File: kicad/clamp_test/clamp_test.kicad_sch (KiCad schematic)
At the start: 26 parts, among them J1 Conn_Coaxial, J2 Conn_Coaxial, J3 Conn_01x03_Pin, J4 Conn_Coaxial, U1 LT1365CS

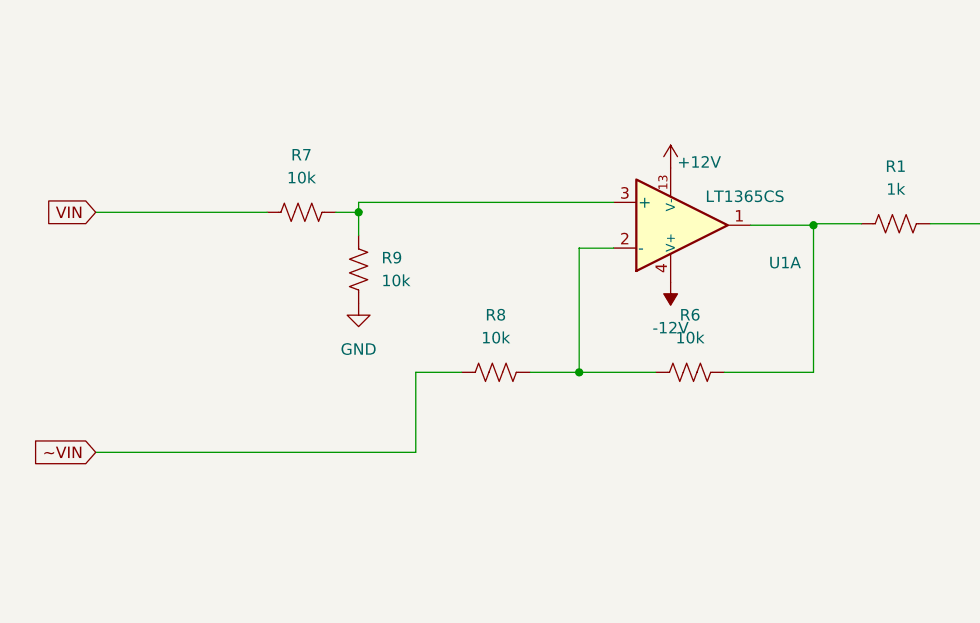
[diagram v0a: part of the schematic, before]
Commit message: adjusted layout
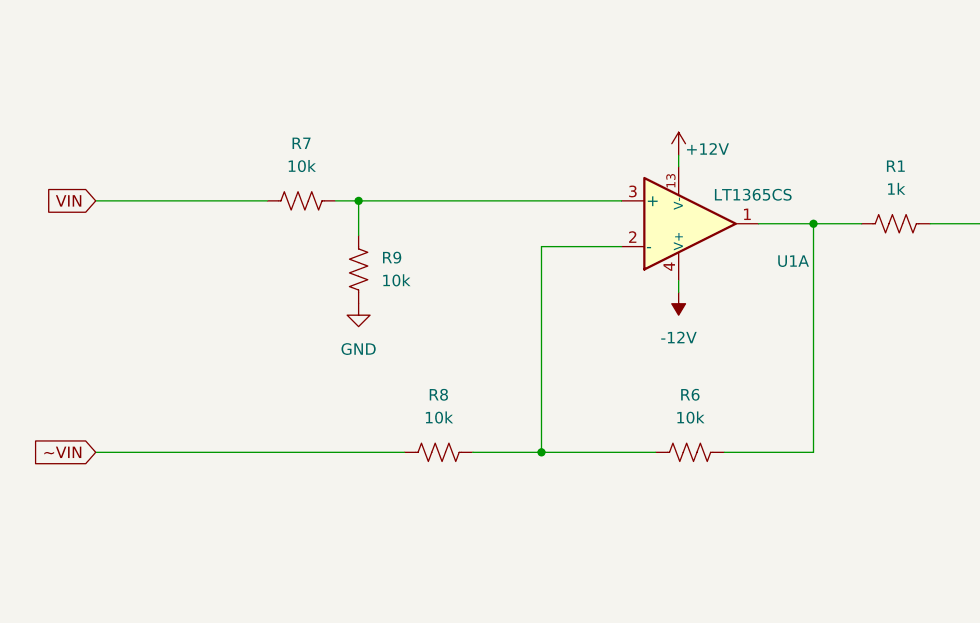
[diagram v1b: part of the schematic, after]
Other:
- moved on the sheet: R6, R7, R8, U1A
